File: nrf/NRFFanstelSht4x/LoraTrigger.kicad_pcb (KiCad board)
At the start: 2 copper layers, 19.8 x 30.3 mm, 12 parts, among them J1 Conn_01x04_Male, J2 Conn_01x04_Male, J3 Conn_01x02_Male, J4 Conn_01x04_Male, U1 BT, U4 SHT4x

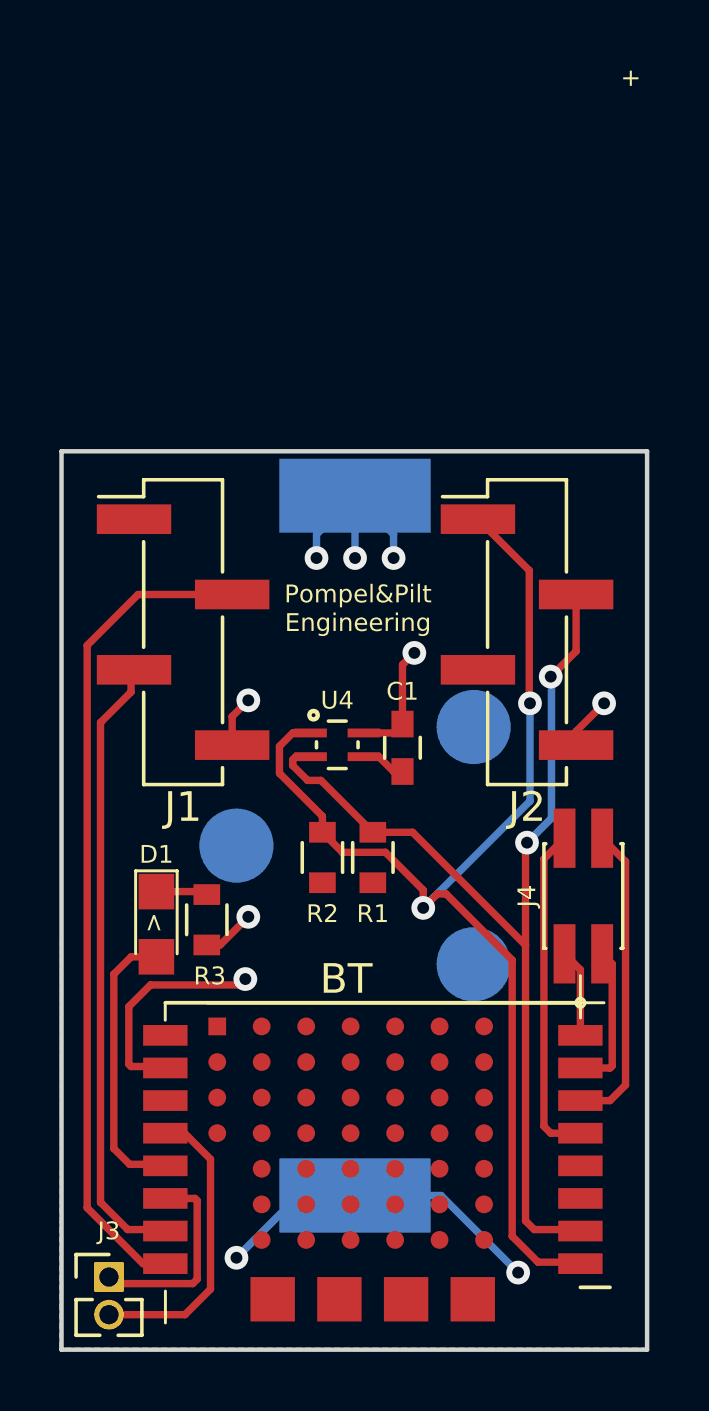
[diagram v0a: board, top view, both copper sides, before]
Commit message: fanstelsht4x prod
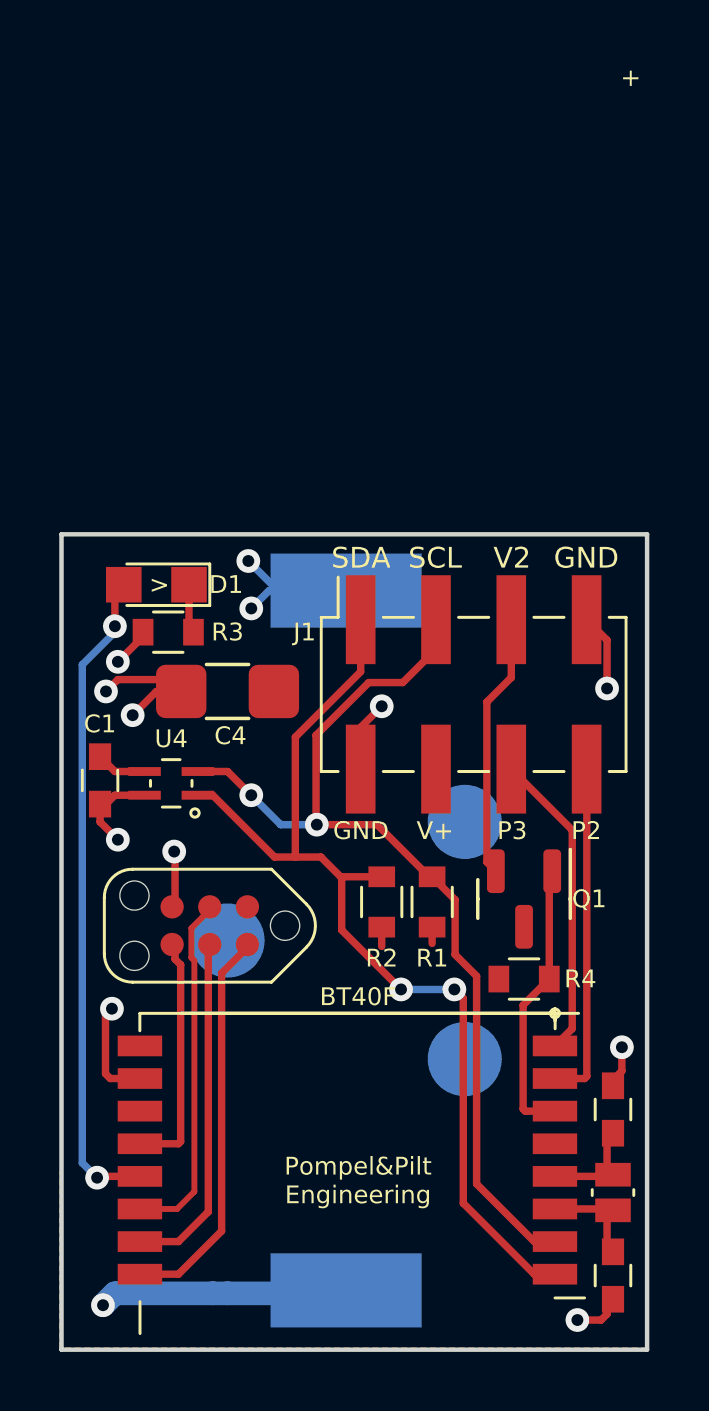
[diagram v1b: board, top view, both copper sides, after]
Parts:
- removed J3: Conn_01x02_Male, Connector_PinHeader_1.27mm:PinHeader_1x02_P1.27mm_Vertical
- removed J4: Conn_01x04_Male, halib:PinHeader_2x02_P1.27mm_Vertical_SMD
- added C2: 10pF, halib:C_0603_Compact_hand, F.Cu at (117.2, 80.1)
- added C3: 10pF, halib:C_0603_Compact_hand, F.Cu at (117.2, 74.5)
- added C4: C106, Capacitor_SMD:C_1206_3216Metric_Pad1.33x1.80mm_HandSolder, F.Cu at (104.2, 60.4)
- added Q1: Q_PMOS_GSD, Package_TO_SOT_SMD:SOT-23, F.Cu at (114.2, 67.4)
- added R4: 100k, halib:R_0603_Compact_hand, F.Cu at (114.2, 70.1)
- added Y1: Crystal_Small, Crystal:Crystal_SMD_MicroCrystal_CM9V-T1A-2Pin_1.6x1.0mm, F.Cu at (117.2, 77.3)
- J1: value Conn_01x04_Male -> Conn_02x04_Odd_Even; footprint Connector_PinHeader_2.54mm:PinHeader_1x04_P2.54mm_Vertical_SMD_Pin1Left -> Connector_PinSocket_2.54mm:PinSocket_2x04_P2.54mm_Vertical_SMD
- J2: value Conn_01x04_Male -> tc2030; footprint Connector_PinHeader_2.54mm:PinHeader_1x04_P2.54mm_Vertical_SMD_Pin1Left -> halib:TC2030
- U1: value BT -> BT40F
- moved J2 14.6 mm to (103.6, 68.3), turned to 180 degrees
- moved D1 11.5 mm to (101.8, 56.8), turned to 180 degrees
- moved C1 10.3 mm to (99.9, 63.4), turned to -90 degrees
- moved J1 10.0 mm to (112.5, 60.5), turned to 90 degrees
- moved R3 9.79 mm to (102.2, 58.4), turned to 180 degrees
- moved U4 5.75 mm to (102.3, 63.5), turned to 180 degrees
- moved BT1 3.21 mm to (108.2, 68.8)
- moved R1 2.50 mm to (111.1, 67.5)
- moved R2 2.50 mm to (109.4, 67.5)
- moved U1 0.93 mm to (115.2, 71.3)
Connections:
- J1 pad 1: VCC -> /SDA
- J1 pad 2: /SWDIO -> GND
- J1 pad 3: /SWDCLK -> /SCL
- J1 pad 4: GND -> VCC
- J2 pad 1: /SDA -> VCC
- J2 pad 2: /SCL -> /SWDIO
- J2 pad 3: VCC -> /RESET
- J2 pad 4: GND -> /SWDCLK
- U1 pad P$3: unconnected-(U1-PadP$3) -> /XL1
- U1 pad P$4: unconnected-(U1-PadP$4) -> /XL2
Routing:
- net /SWDIO: track 28.0 -> 13.1 mm
- net /LED: track 8.96 -> 22.3 mm, vias 0 -> 2
- net /P004: track 11.3 -> 0.00 mm
- net /V2: track 0.00 -> 8.95 mm
- net /SWDCLK: track 20.4 -> 11.5 mm
- net /P003: track 2.97 -> 10.4 mm
- net /SDA: track 41.3 -> 34.4 mm
- net /P002: track 5.02 -> 11.5 mm
- net GND: track 16.6 -> 22.8 mm, vias 5 -> 10
- net /RESET: track 6.88 -> 11.7 mm
- net /XL2: track 0.00 -> 3.18 mm
- net /XL1: track 0.00 -> 3.18 mm
- net VCC: track 20.8 -> 18.4 mm, vias 5 -> 3
- net /SWO: track 10.1 -> 7.83 mm
- net /SCL: track 35.3 -> 33.4 mm
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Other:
- board size 19.8 x 30.3 mm -> 19.8 x 27.5 mm
- board text added: "GND"
- board text added: "P2"
- board text added: "P3"
- board text added: "SCL"
- board text added: "SDA"
- board text added: "V+"
- board text added: "V2"
